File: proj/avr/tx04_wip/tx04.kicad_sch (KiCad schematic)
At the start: 14 parts, among them J1 Conn_02x10_Counter_Clockwise, J2 USB_C_Receptacle_USB2.0_16P, SW1 SW_Push, U1 ATtiny1606-M, U2 CH340E, U3 TS5A23159DGS

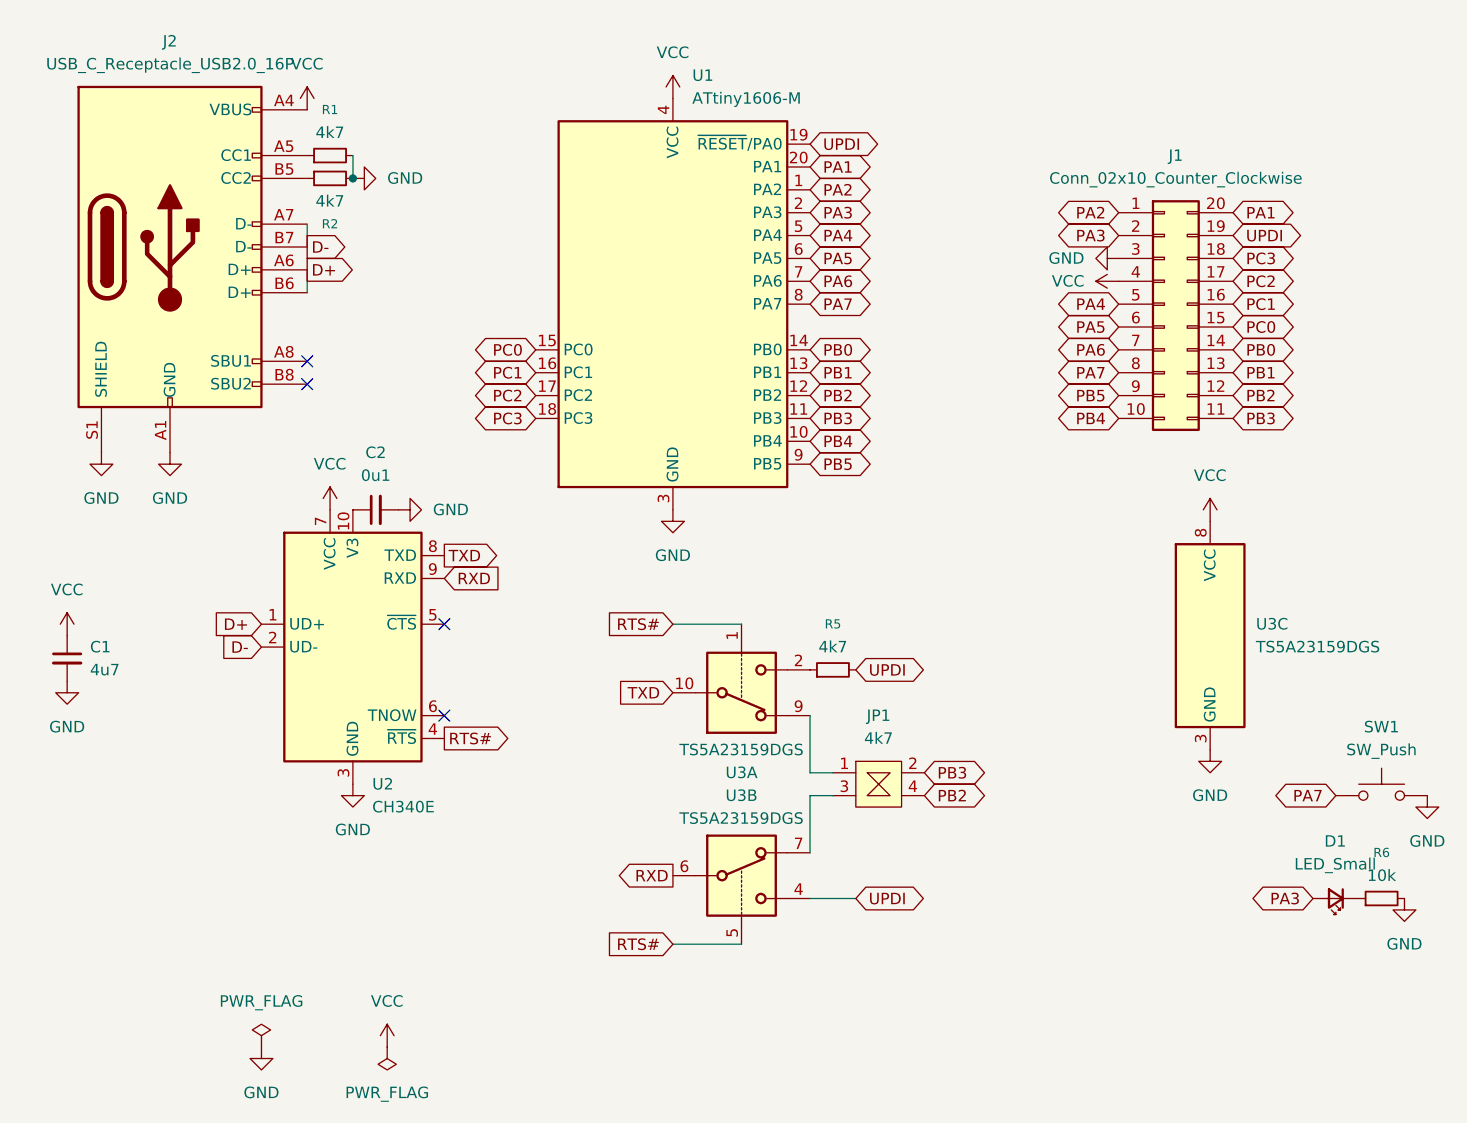
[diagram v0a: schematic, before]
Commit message: -
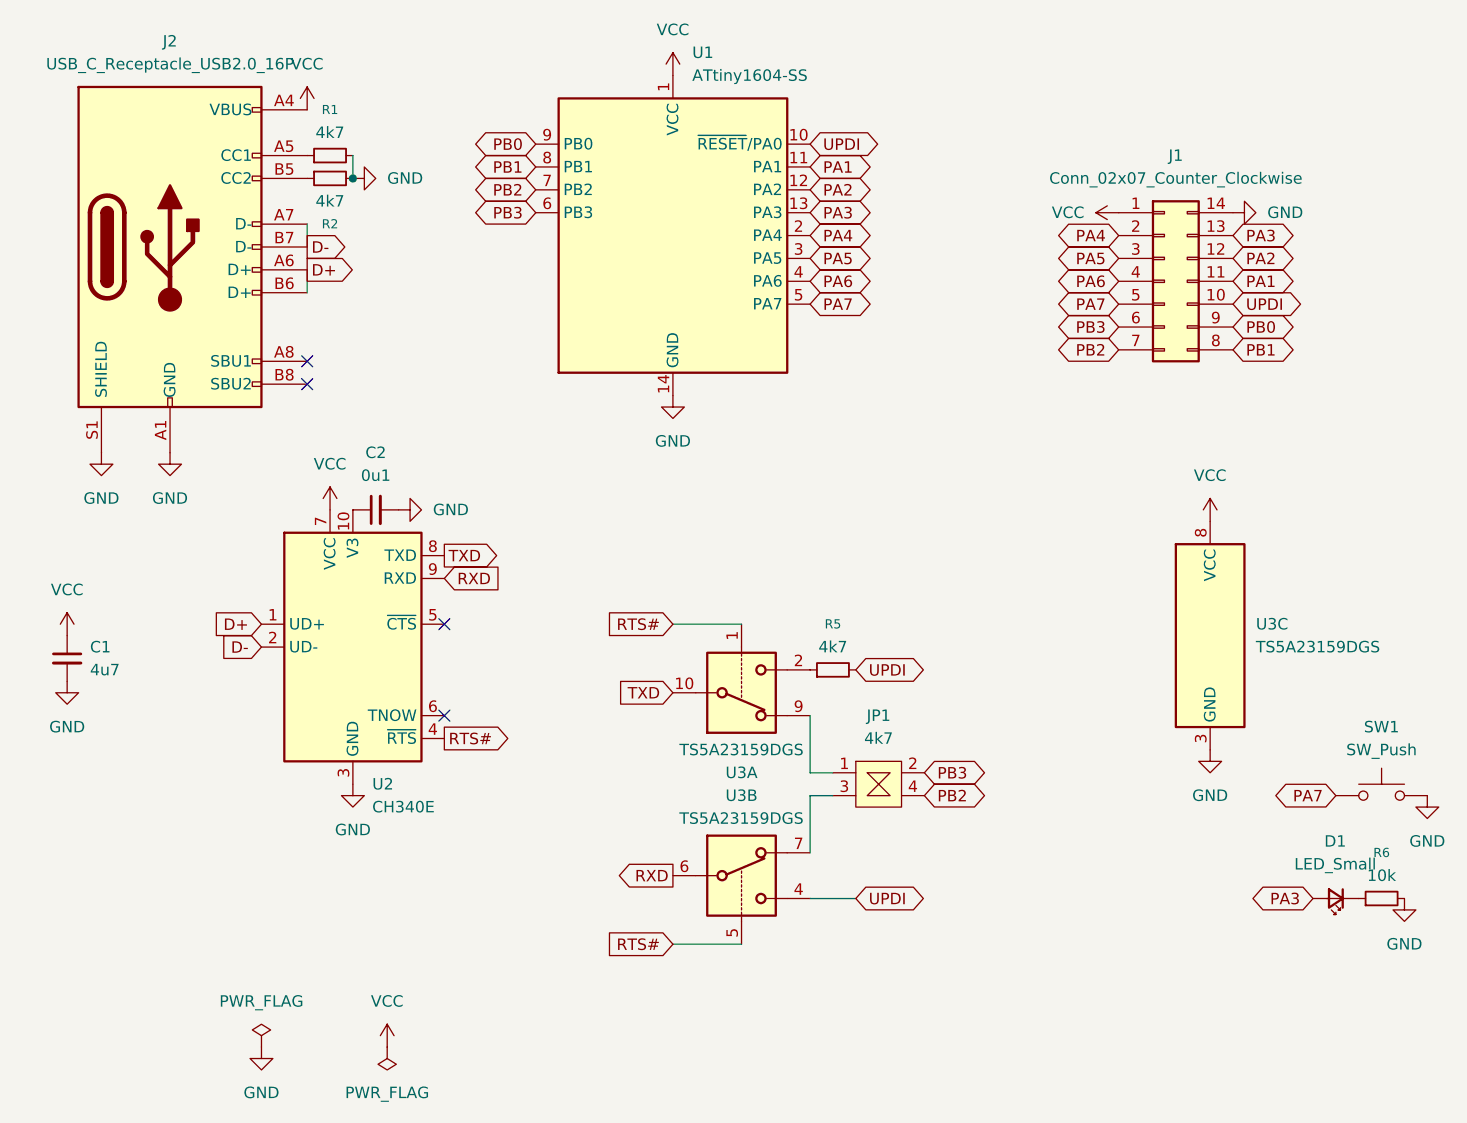
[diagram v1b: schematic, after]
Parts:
- removed J1: Conn_02x10_Counter_Clockwise, Package_DIP:DIP-20_W7.62mm_Socket, symbol Connector_Generic:Conn_02x10_Counter_Clockwise
- removed U1: ATtiny1606-M, Package_DFN_QFN:VQFN-20-1EP_3x3mm_P0.4mm_EP1.7x1.7mm, symbol MCU_Microchip_ATtiny:ATtiny1606-M
- added J1: Conn_02x07_Counter_Clockwise, Package_DIP:DIP-14_W10.16mm, symbol Connector_Generic:Conn_02x07_Counter_Clockwise
- added U1: ATtiny1604-SS, Package_SO:SOIC-14_3.9x8.7mm_P1.27mm, symbol MCU_Microchip_ATtiny:ATtiny1604-SS
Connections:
- net GND: now also J1.14 (Pin_14), U1.14 (GND)
- net PA1: now also J1.11 (Pin_11), U1.11 (PA1)
- net PA2: now also J1.12 (Pin_12), U1.12 (PA2)
- net PA3: now also J1.13 (Pin_13), U1.13 (PA3)
- net PA4: now also J1.2 (Pin_2), U1.2 (PA4)
- net PA5: now also J1.3 (Pin_3), U1.3 (PA5)
- net PA6: now also J1.4 (Pin_4), U1.4 (PA6)
- net PA7: now also J1.5 (Pin_5), U1.5 (PA7)
- net PB0: now also J1.9 (Pin_9), U1.9 (PB0)
- net PB1: now also J1.8 (Pin_8), U1.8 (PB1)
- net PB2: now also J1.7 (Pin_7), U1.7 (PB2)
- net PB3: now also J1.6 (Pin_6), U1.6 (PB3)
- net UPDI: now also J1.10 (Pin_10), U1.10 (~{RESET}/PA0)
- net VCC: now also J1.1 (Pin_1), U1.1 (VCC)

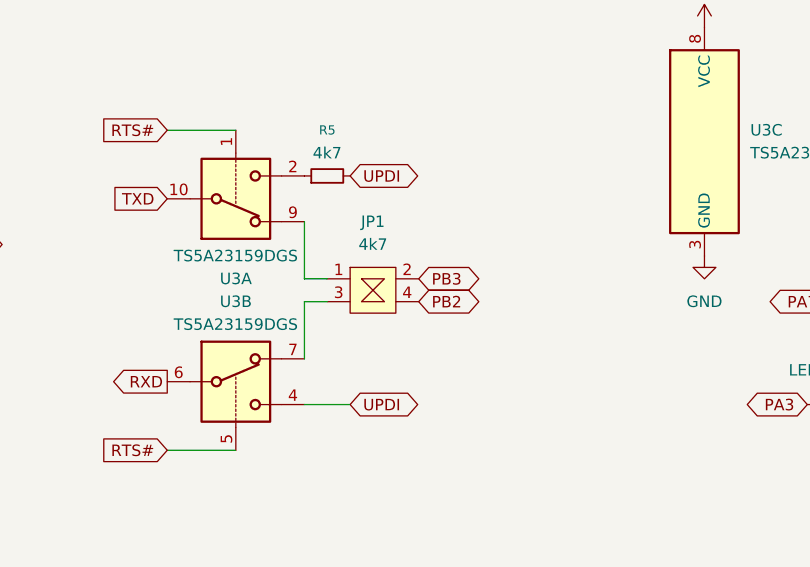
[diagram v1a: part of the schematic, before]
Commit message: -
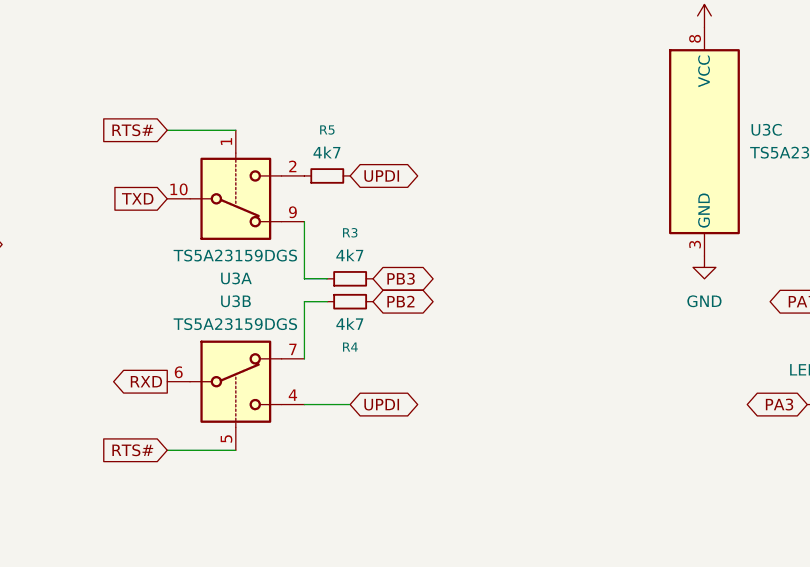
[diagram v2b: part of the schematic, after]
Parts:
- removed JP1: 4k7, Library:pokayoke_1608, symbol Library:pokayoke
- added R3, R4: 4k7, Resistor_SMD:R_0603_1608Metric, symbol Device:R_Small
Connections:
- net PB2: now also R4.2
- net PB3: now also R3.2
- net at U3.9: now also R3.1
- net at U3.7: now also R4.1
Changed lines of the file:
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@@
 	(global_label "PB2"
 		(shape bidirectional)
-		(at 118.11 137.16 0)
+		(at 113.03 137.16 0)
 		(fields_autoplaced yes)
 		(effects
@@
 		)
 		(property "Intersheetrefs" "${INTERSHEET_REFS}"
-			(at 125.956 137.16 0)
+			(at 120.876 137.16 0)
 			(effects
 				(font
@@
 	(global_label "PB3"
 		(shape bidirectional)
-		(at 118.11 134.62 0)
+		(at 113.03 134.62 0)
 		(fields_autoplaced yes)
 		(effects
@@
 		)
 		(property "Intersheetrefs" "${INTERSHEET_REFS}"
-			(at 125.956 134.62 0)
+			(at 120.876 134.62 0)
 			(effects
 				(font
@@
 	)
 	(symbol
+		(lib_id "Device:R_Small")
+		(at 110.49 137.16 90)
+		(mirror x)
+		(unit 1)
+		(exclude_from_sim no)
+		(in_bom yes)
+		(on_board yes)
+		(dnp no)
+		(property "Reference" "R4"
+			(at 110.49 142.24 90)
+			(effects
+				(font
+					(size 1.016 1.016)
+				)
+			)
+		)
+		(property "Value" "4k7"
+			(at 110.49 139.7 90)
+			(effects
+				(font
+					(size 1.27 1.27)
+				)
+			)
+		)
+		(property "Footprint" "Resistor_SMD:R_0603_1608Metric"
+			(at 110.49 137.16 0)
+			(effects
+				(font
+					(size 1.27 1.27)
+				)
+				(hide yes)
+			)
+		)
+		(property "Datasheet" "~"
+			(at 110.49 137.16 0)
+			(effects
+				(font
+					(size 1.27 1.27)
+				)
+				(hide yes)
+			)
+		)
+		(property "Description" "Resistor, small symbol"
+			(at 110.49 137.16 0)
+			(effects
+				(font
+					(size 1.27 1.27)
+				)
+				(hide yes)
+			)
+		)
+		(pin "2"
+		)
+		(pin "1"
+		)
+		(instances
+			(project "tx04"
+				(path "/73158485-b41d-4a6f-a576-c7b38822ce40"
+					(reference "R4")
+					(unit 1)
+				)
+			)
+		)
+	)
+	(symbol
 		(lib_id "power:GND")
 		(at 54.61 68.58 90)
@@
 	)
 	(symbol
-		(lib_id "Library:pokayoke")
-		(at 111.76 134.62 0)
-		(unit 1)
-		(exclude_from_sim no)
-		(in_bom yes)
-		(on_board yes)
-		(dnp no)
-		(fields_autoplaced yes)
-		(property "Reference" "JP1"
-			(at 113.03 128.27 0)
-			(effects
-				(font
-					(size 1.27 1.27)
-				)
-			)
-		)
-		(property "Value" "4k7"
-			(at 113.03 130.81 0)
-			(effects
-				(font
-					(size 1.27 1.27)
-				)
-			)
-		)
-		(property "Footprint" "Library:pokayoke_1608"
-			(at 111.76 134.62 0)
-			(effects
-				(font
-					(size 1.27 1.27)
-				)
-				(hide yes)
-			)
-		)
-		(property "Datasheet" ""
-			(at 111.76 134.62 0)
-			(effects
-				(font
-					(size 1.27 1.27)
-				)
-				(hide yes)
-			)
-		)
-		(property "Description" ""
-			(at 111.76 134.62 0)
-			(effects
-				(font
-					(size 1.27 1.27)
-				)
-				(hide yes)
-			)
-		)
-		(pin "1"
-		)
-		(pin "4"
-		)
-		(pin "2"
-		)
-		(pin "3"
-		)
-		(instances
-			(project ""
-				(path "/73158485-b41d-4a6f-a576-c7b38822ce40"
-					(reference "JP1")
-					(unit 1)
-				)
-			)
-		)
-	)
-	(symbol
 		(lib_id "Connector:USB_C_Receptacle_USB2.0_16P")
 		(at 34.29 76.2 0)
@@
 					(unit 1)
 				)
+			)
+		)
+	)
+	(symbol
+		(lib_id "Device:R_Small")
+		(at 110.49 134.62 90)
+		(unit 1)
+		(exclude_from_sim no)
+		(in_bom yes)
+		(on_board yes)
+		(dnp no)
+		(property "Reference" "R3"
+			(at 110.49 129.54 90)
+			(effects
+				(font
+					(size 1.016 1.016)
+				)
+			)
+		)
+		(property "Value" "4k7"
+			(at 110.49 132.08 90)
+			(effects
+				(font
+					(size 1.27 1.27)
+				)
+			)
+		)
+		(property "Footprint" "Resistor_SMD:R_0603_1608Metric"
+			(at 110.49 134.62 0)
+			(effects
+				(font
+					(size 1.27 1.27)
+				)
+				(hide yes)
+			)
+		)
+		(property "Datasheet" "~"
+			(at 110.49 134.62 0)
+			(effects
+				(font
+					(size 1.27 1.27)
+				)
+				(hide yes)
+			)
+		)
+		(property "Description" "Resistor, small symbol"
+			(at 110.49 134.62 0)
+			(effects
+				(font
+					(size 1.27 1.27)
+				)
+				(hide yes)
+			)
+		)
+		(pin "2"
+		)
+		(pin "1"
+		)
+		(instances
+			(project "tx04"
+				(path "/73158485-b41d-4a6f-a576-c7b38822ce40"
+					(reference "R3")
+					(unit 1)
+				)
